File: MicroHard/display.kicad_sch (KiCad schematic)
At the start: 4 parts, among them U6 MAX6955AAX+

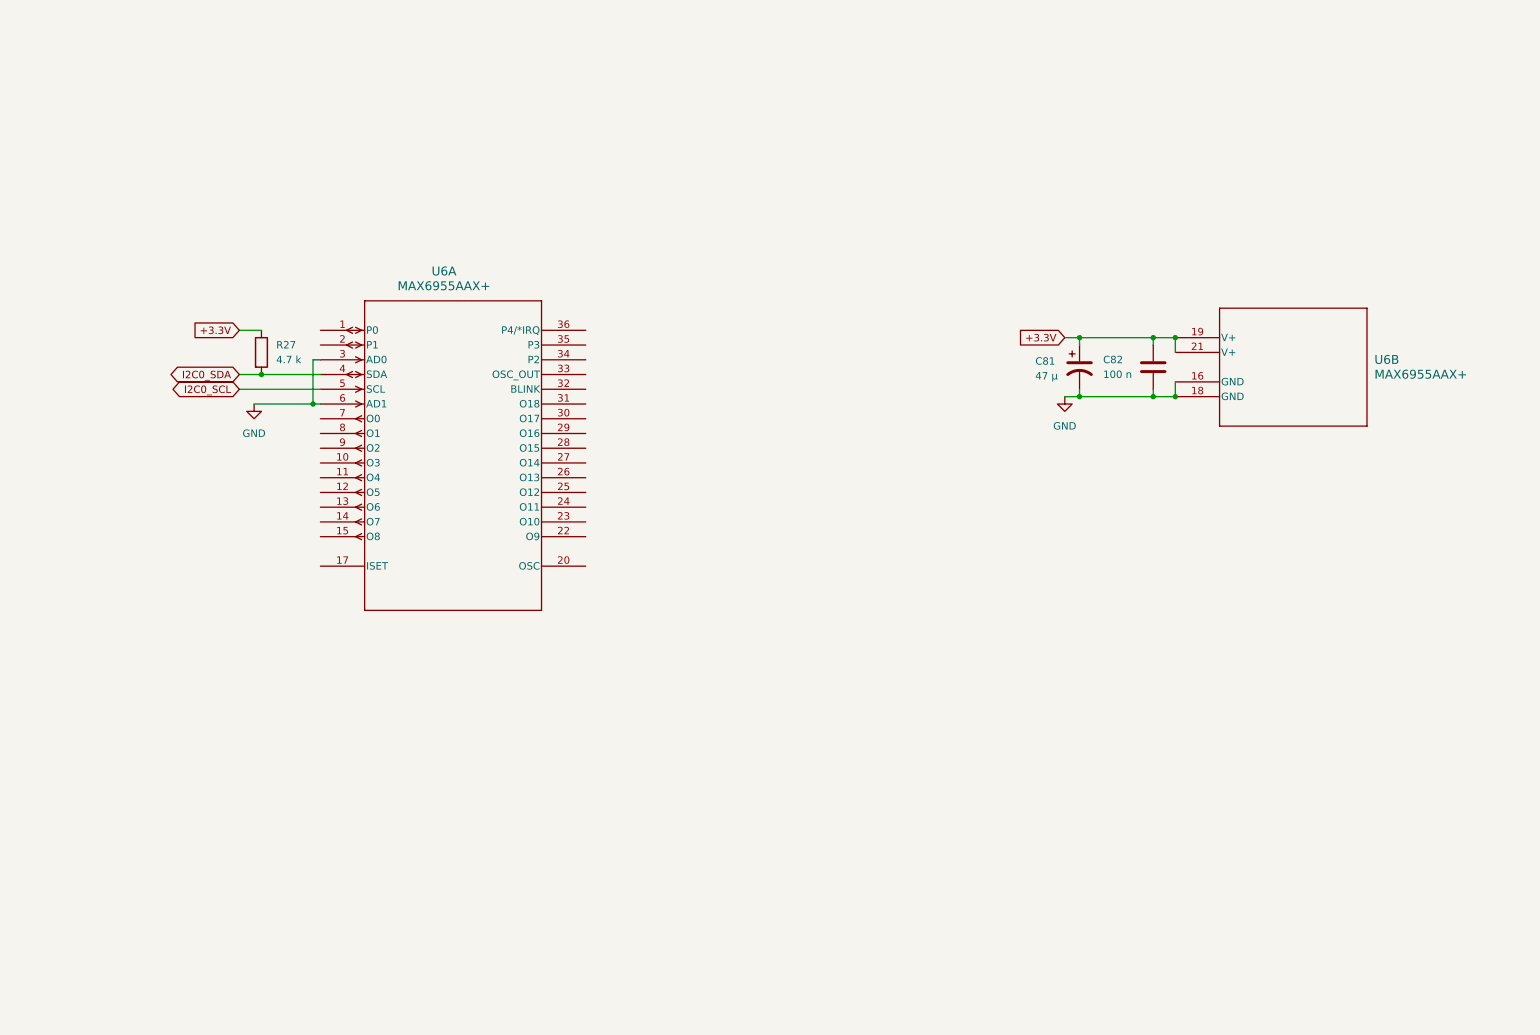
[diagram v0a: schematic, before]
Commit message: Finish display
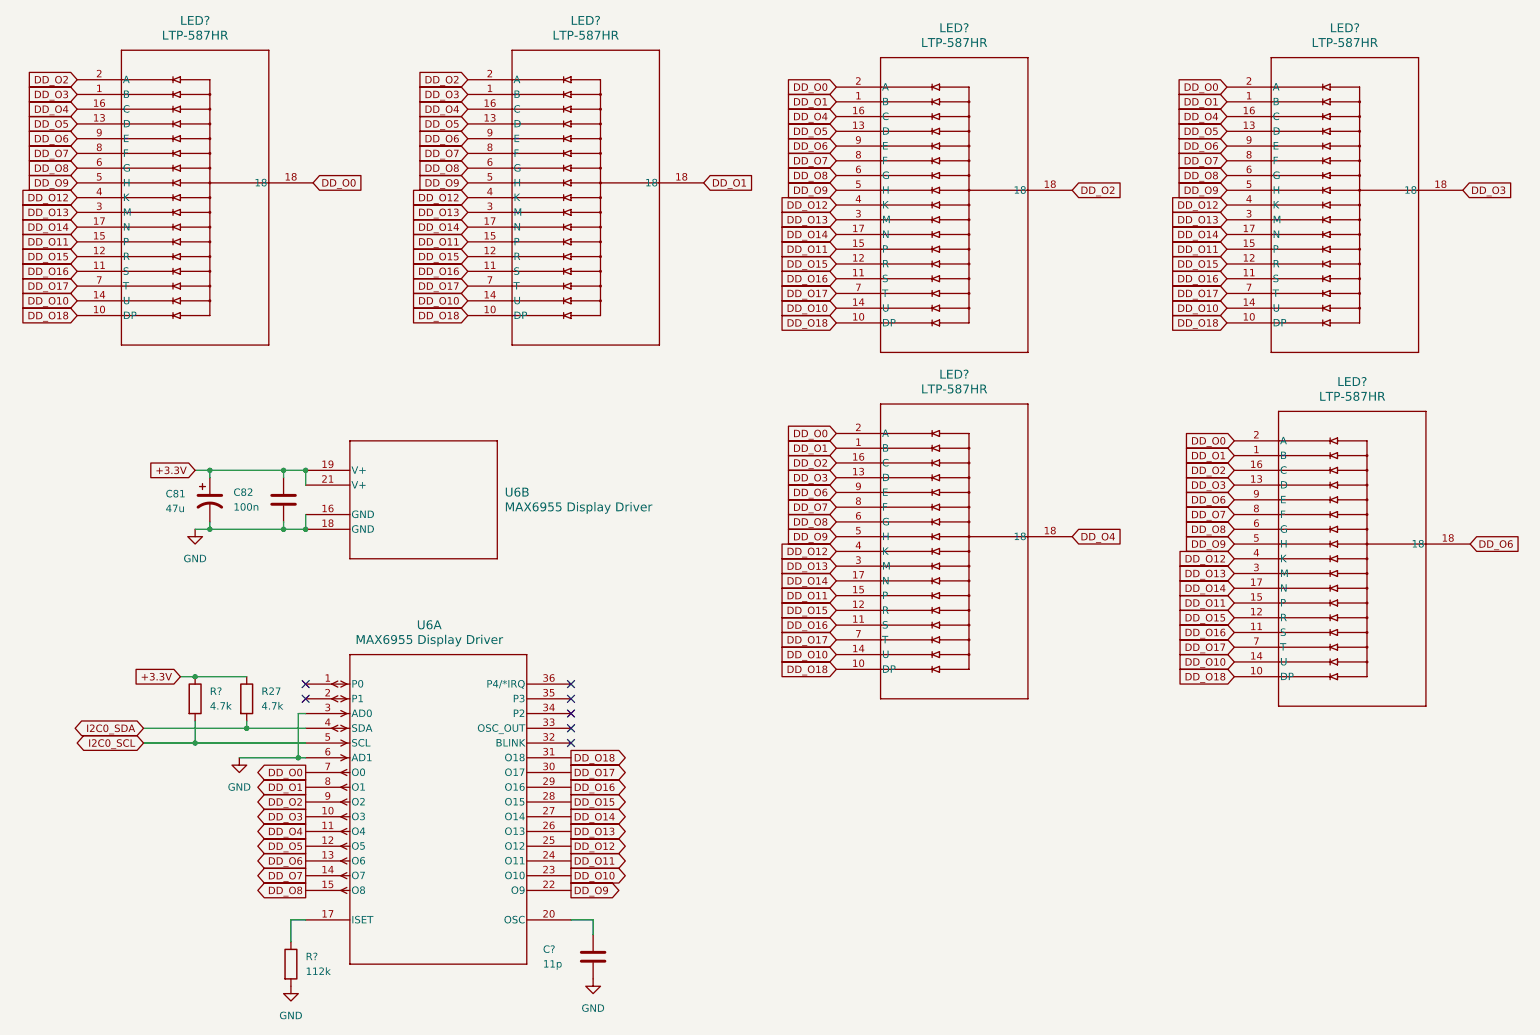
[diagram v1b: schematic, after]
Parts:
- added C?: 11p, symbol Device:C
- added LED? (x6): LTP-587HR, LTP-587HR_LTO, symbol LTP-587HR:LTP-587HR
- added R?: 112k, symbol Device:R
- added R?: 4.7k, Resistor_SMD:R_0805_2012Metric_Pad1.20x1.40mm_HandSolder, symbol Device:R
- C81: value 47 µ -> 47u
- C82: value 100 n -> 100n
- R27: value 4.7 k -> 4.7k; footprint (none) -> Resistor_SMD:R_0805_2012Metric_Pad1.20x1.40mm_HandSolder
- U6: value MAX6955AAX+ -> MAX6955 Display Driver
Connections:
- net +3.3V: now also R?.1
- net GND: now also C?.2, R?.2
- net I2C0_SCL: now also R?.2
- net DD_O3: now reaches U6.10 (O3)
- net DD_O3: now also LED?.1 (B), LED?.1 (B), LED?.13 (D), LED?.13 (D), LED?.18
- net DD_O4: now reaches U6.11 (O4)
- net DD_O4: now also LED?.16 (C), LED?.16 (C), LED?.16 (C), LED?.16 (C), LED?.18
- net DD_O5: now reaches U6.12 (O5)
- net DD_O5: now also LED?.13 (D), LED?.13 (D), LED?.13 (D), LED?.13 (D)
- net DD_O6: now reaches U6.13 (O6)
- net DD_O6: now also LED?.18, LED?.9 (E), LED?.9 (E), LED?.9 (E), LED?.9 (E), LED?.9 (E), LED?.9 (E)
- net DD_O7: now reaches U6.14 (O7)
- net DD_O7: now also LED?.8 (F), LED?.8 (F), LED?.8 (F), LED?.8 (F), LED?.8 (F), LED?.8 (F)
- net DD_O8: now reaches U6.15 (O8)
- net DD_O8: now also LED?.6 (G), LED?.6 (G), LED?.6 (G), LED?.6 (G), LED?.6 (G), LED?.6 (G)
- net at U6.17 (ISET): now also R?.1
- net at U6.20 (OSC): now also C?.1
- net DD_O9: now reaches U6.22 (O9)
- net DD_O9: now also LED?.5 (H), LED?.5 (H), LED?.5 (H), LED?.5 (H), LED?.5 (H), LED?.5 (H)
- net DD_O10: now reaches U6.23 (O10)
- net DD_O10: now also LED?.14 (U), LED?.14 (U), LED?.14 (U), LED?.14 (U), LED?.14 (U), LED?.14 (U)
- net DD_O11: now reaches U6.24 (O11)
- net DD_O11: now also LED?.15 (P), LED?.15 (P), LED?.15 (P), LED?.15 (P), LED?.15 (P), LED?.15 (P)
- net DD_O12: now reaches U6.25 (O12)
- net DD_O12: now also LED?.4 (K), LED?.4 (K), LED?.4 (K), LED?.4 (K), LED?.4 (K), LED?.4 (K)
- net DD_O13: now reaches U6.26 (O13)
- net DD_O13: now also LED?.3 (M), LED?.3 (M), LED?.3 (M), LED?.3 (M), LED?.3 (M), LED?.3 (M)
- net DD_O14: now reaches U6.27 (O14)
- net DD_O14: now also LED?.17 (N), LED?.17 (N), LED?.17 (N), LED?.17 (N), LED?.17 (N), LED?.17 (N)
- net DD_O15: now reaches U6.28 (O15)
- net DD_O15: now also LED?.12 (R), LED?.12 (R), LED?.12 (R), LED?.12 (R), LED?.12 (R), LED?.12 (R)
- net DD_O16: now reaches U6.29 (O16)
- net DD_O16: now also LED?.11 (S), LED?.11 (S), LED?.11 (S), LED?.11 (S), LED?.11 (S), LED?.11 (S)
- net DD_O17: now reaches U6.30 (O17)
- net DD_O17: now also LED?.7 (T), LED?.7 (T), LED?.7 (T), LED?.7 (T), LED?.7 (T), LED?.7 (T)
- net DD_O18: now reaches U6.31 (O18)
- net DD_O18: now also LED?.10 (DP), LED?.10 (DP), LED?.10 (DP), LED?.10 (DP), LED?.10 (DP), LED?.10 (DP)
- net DD_O0: now reaches U6.7 (O0)
- net DD_O0: now also LED?.18, LED?.2 (A), LED?.2 (A), LED?.2 (A), LED?.2 (A)
- net DD_O1: now reaches U6.8 (O1)
- net DD_O1: now also LED?.1 (B), LED?.1 (B), LED?.1 (B), LED?.1 (B), LED?.18
- net DD_O2: now reaches U6.9 (O2)
- net DD_O2: now also LED?.16 (C), LED?.16 (C), LED?.18, LED?.2 (A), LED?.2 (A)
- no-connect marks 0 -> 7
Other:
- moved on the sheet: C81, C82, R27, U6A, U6B
